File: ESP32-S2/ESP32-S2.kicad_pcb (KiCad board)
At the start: 4 copper layers, 27.8 x 70.3 mm, 45 parts, among them IC1 IP4220CZ6, J1 USB_A, J2 TYPE-C-31-M-12, J3 Conn_01x18_Male, J4 S2B-PH-SM4-TB(LF)(SN), J5 Conn_01x22_Male, SW1 SW_Push, SW2 SW_Push, U1 ESP32-S2-WROOM-ESP32-S2-WROOM, U2 MMBT8050, U3 MMBT8050, U4 MCP73831-2-OT, U5 AMS1117-3.3, U6 CH340C

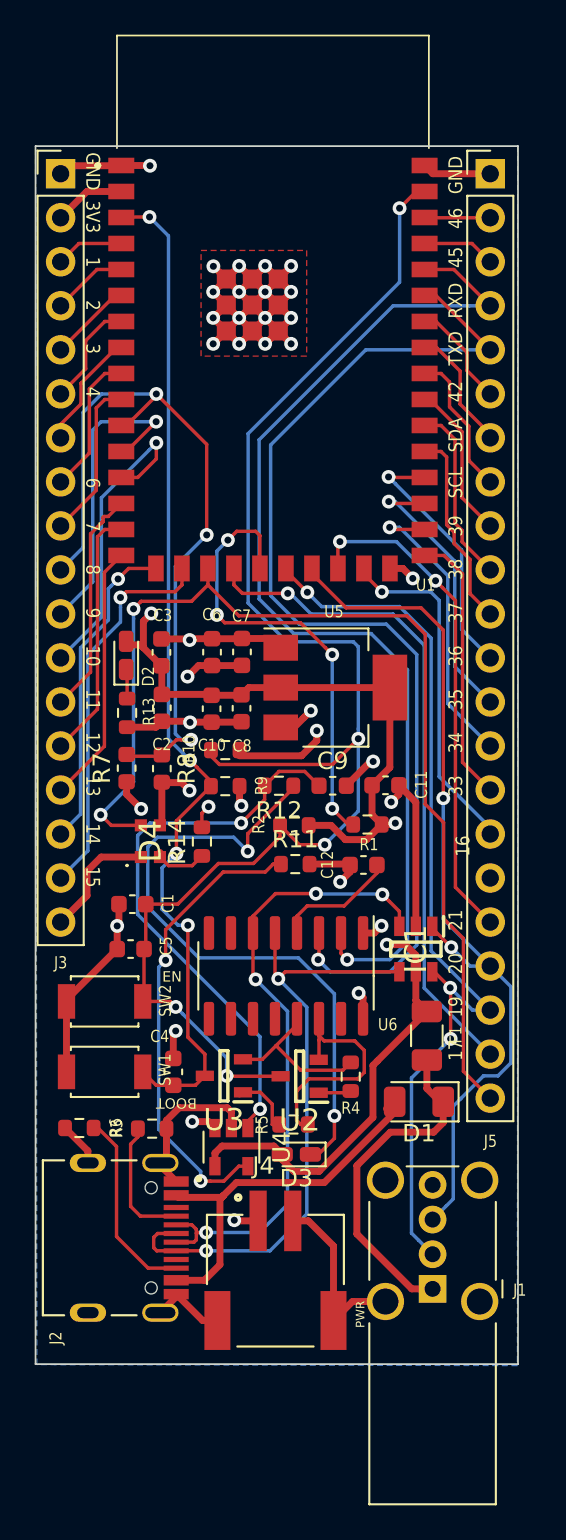
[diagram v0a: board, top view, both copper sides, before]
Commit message: Minor Changes
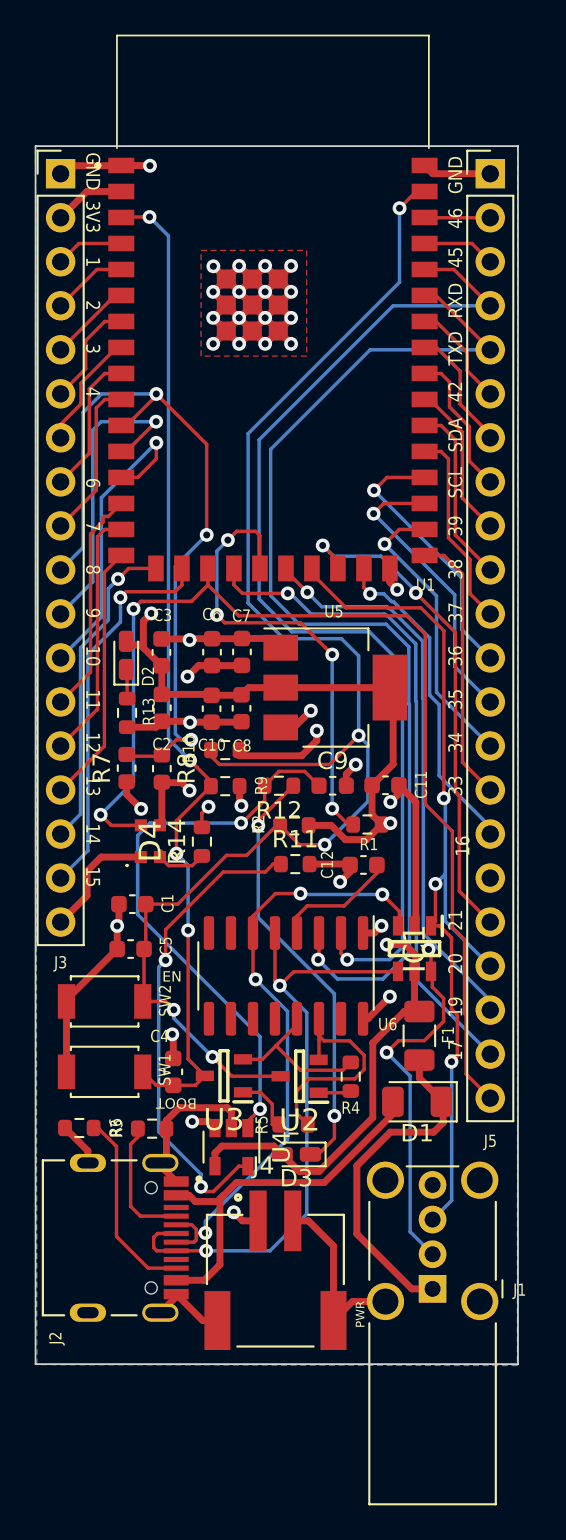
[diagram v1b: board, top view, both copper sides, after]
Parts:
- moved F1 0.43 mm to (159.2, 118.4)
- moved D1 0.10 mm to (159.0, 122.2)
- moved IC1 0.08 mm to (158.9, 113.4)
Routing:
- net Net-(D3-Pad1): track 37.6 -> 24.8 mm
- net /DN1: track 36.9 -> 35.2 mm
- net /GPIO26: track 20.0 -> 18.9 mm
- net /GPIO0: track 59.5 -> 58.4 mm
- net GND: track 123.7 -> 123.0 mm
- net /GPIO36: track 15.0 -> 15.7 mm
- net Net-(R11-Pad1): track 27.0 -> 27.7 mm
- net /GPIO34: track 17.4 -> 16.8 mm
- net /GPIO35: track 16.3 -> 16.8 mm
- net /CHIP_PU: track 86.4 -> 85.8 mm
- net /~RTS: track 14.4 -> 13.8 mm
- net /GPIO20: track 51.8 -> 51.7 mm, vias 2 -> 3
